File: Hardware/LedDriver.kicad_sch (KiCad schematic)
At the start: 10 parts, among them J1 Connector_4p, U1 AP3019A

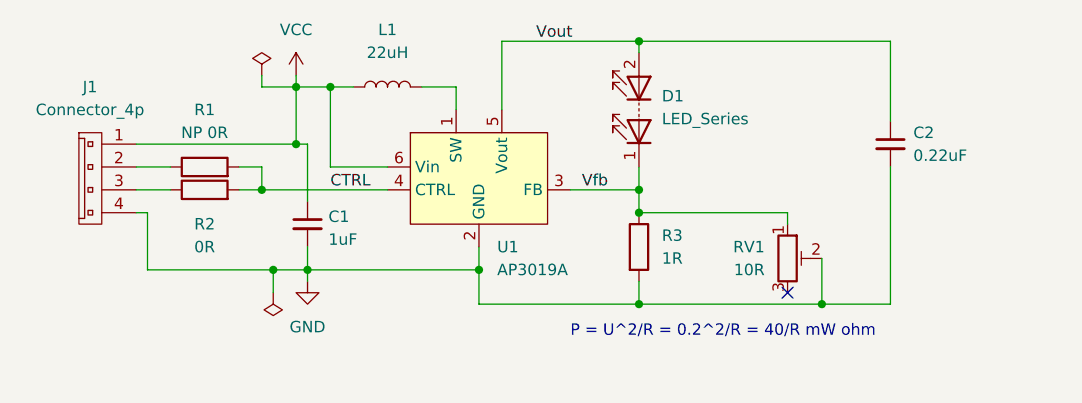
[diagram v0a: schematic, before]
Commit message: edited libraries
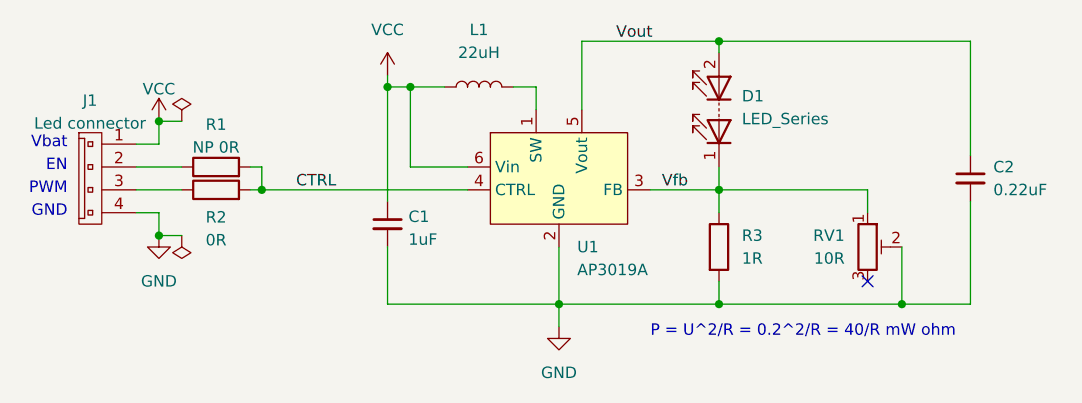
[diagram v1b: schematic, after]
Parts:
- J1: value Connector_4p -> Led connector; footprint 0ESN_Lib:Connector_2p_m -> 0ESN_Lib:Connector_4p_m
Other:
- note added: "EN"
- note added: "GND"
- note added: "PWM"
- note added: "Vbat"
- moved on the sheet: C1, C2, D1, L1, R1, R2, R3, RV1, U1
